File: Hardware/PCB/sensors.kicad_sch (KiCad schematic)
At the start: 26 parts, among them IC3 MPX5500DP, IC4 MPX5500DP, U2 ADS1219IPWR, U6 TPS7A2050PDBVR

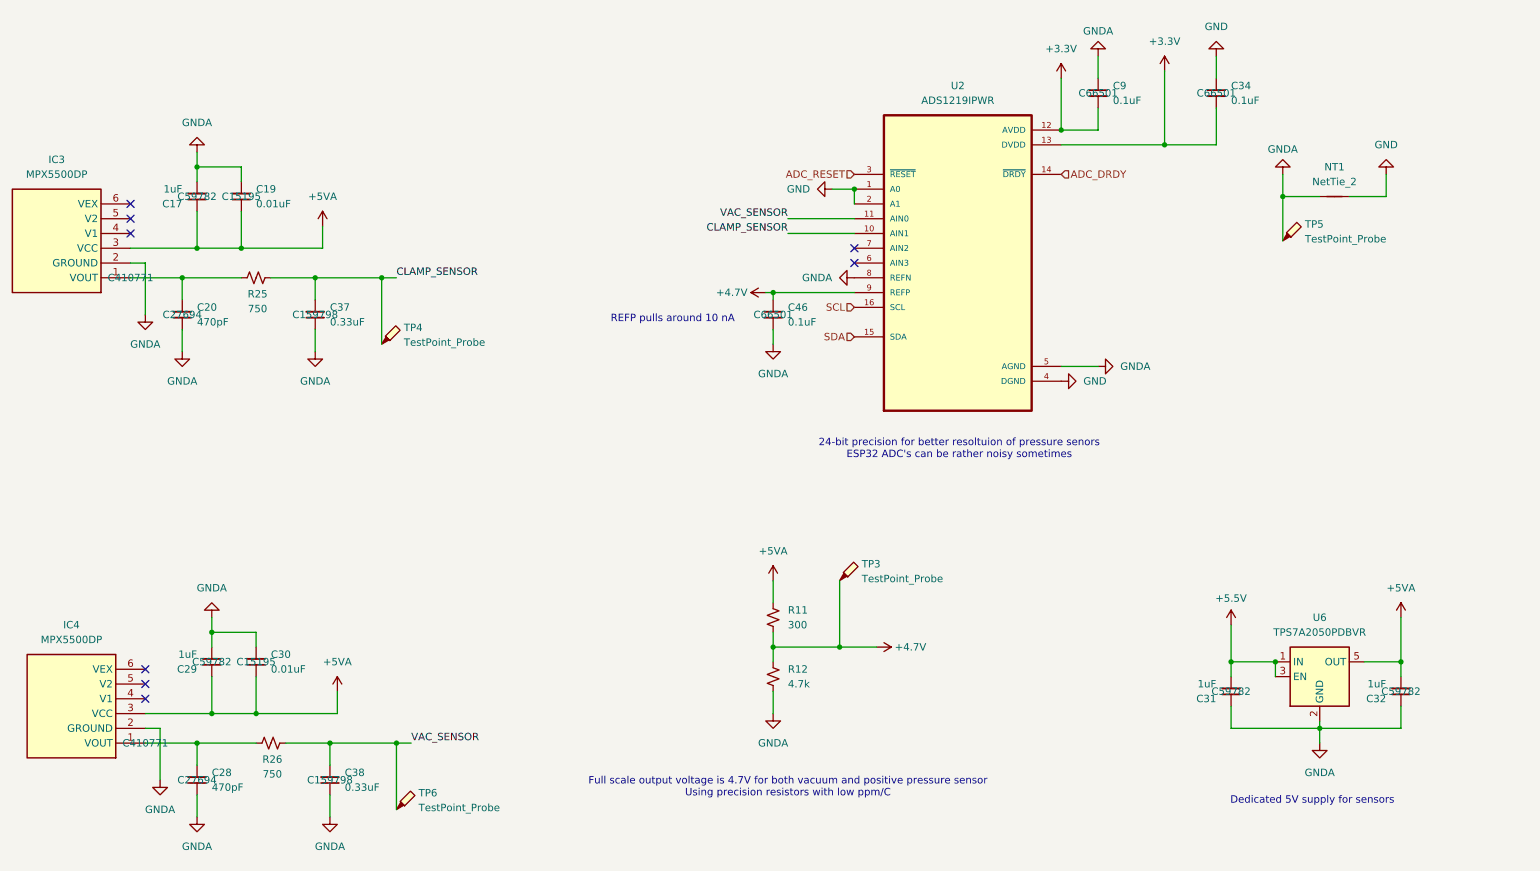
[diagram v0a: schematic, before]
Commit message: done with this, placed order
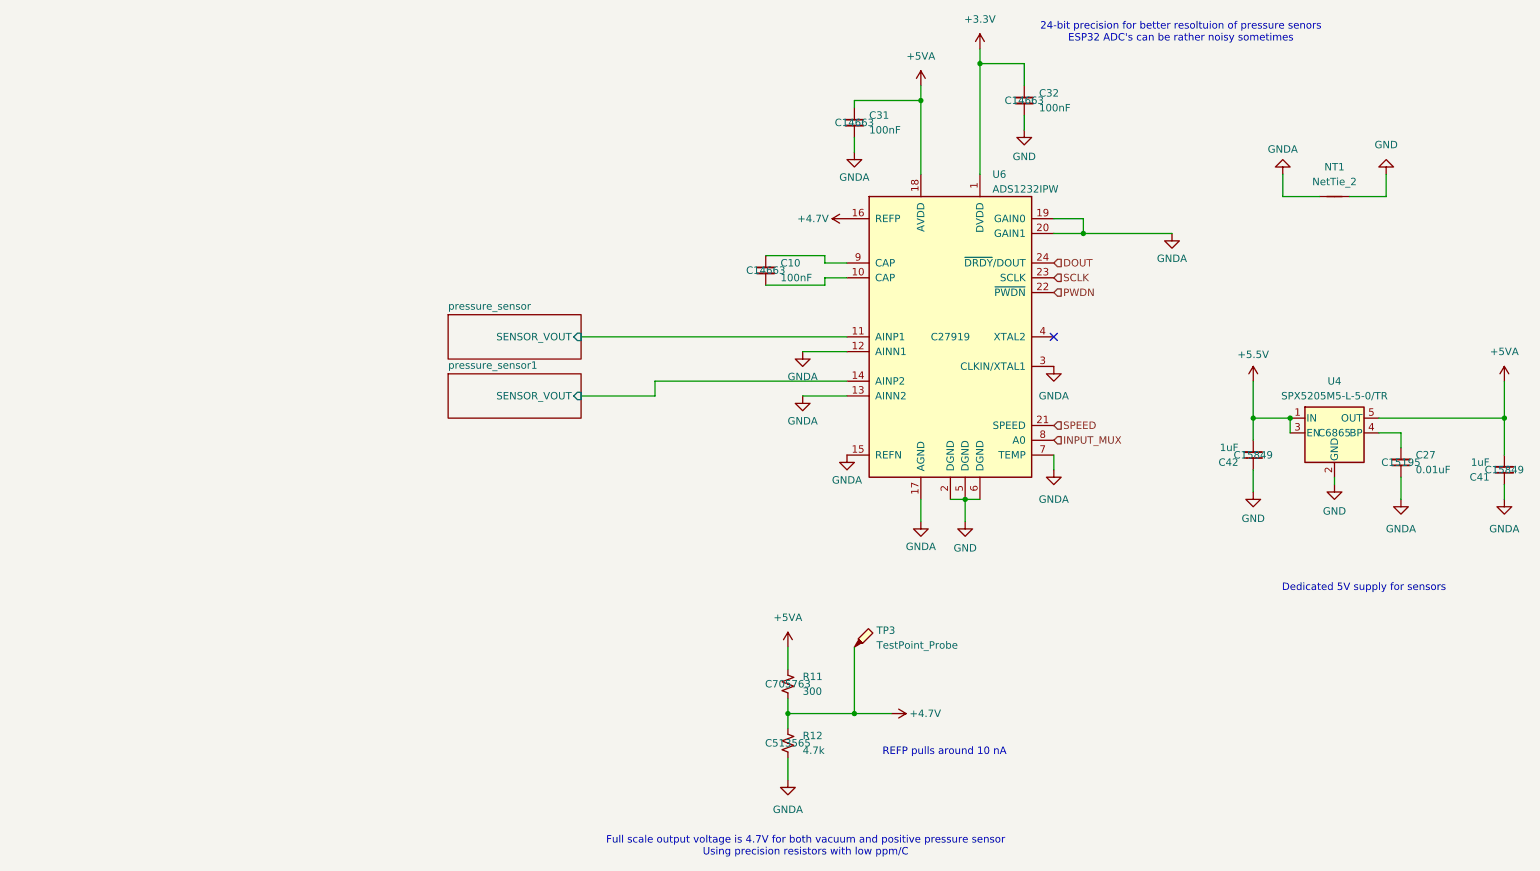
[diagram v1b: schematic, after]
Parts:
- removed C17, C29: 1uF, Capacitor_SMD:C_0603_1608Metric_Pad1.08x0.95mm_HandSolder, symbol Device:C_Small
- removed C19, C30: 0.01uF, Capacitor_SMD:C_0402_1005Metric_Pad0.74x0.62mm_HandSolder, symbol Device:C_Small
- removed C20, C28: 470pF, Capacitor_SMD:C_0603_1608Metric_Pad1.08x0.95mm_HandSolder, symbol Device:C_Small
- removed C34, C46, C9: 0.1uF, Capacitor_SMD:C_0603_1608Metric_Pad1.08x0.95mm_HandSolder, symbol Device:C_Small
- removed C37, C38: 0.33uF, Capacitor_SMD:C_0603_1608Metric_Pad1.08x0.95mm_HandSolder, symbol Device:C_Small
- removed IC3, IC4: MPX5500DP, Vendor_Footprints:MPX5500DP, symbol Vendor_Symbols:MPX5500DP
- removed R25, R26: 750, Resistor_SMD:R_0603_1608Metric_Pad0.98x0.95mm_HandSolder, symbol Device:R_Small_US
- removed TP4, TP5, TP6: TestPoint_Probe, TestPoint:TestPoint_Keystone_5000-5004_Miniature, symbol Connector:TestPoint_Probe
- removed U2: ADS1219IPWR, Vendor_Footprints:SOP65P640X120-16N, symbol Vendor_Symbols:ADS1219IPWR
- removed U6: TPS7A2050PDBVR, Package_TO_SOT_SMD:SOT-23-5, symbol Regulator_Linear:TPS7A0531PDBV
- added C10: 100nF, Capacitor_SMD:C_0603_1608Metric_Pad1.08x0.95mm_HandSolder, symbol Device:C_Small
- added C27: 0.01uF, Capacitor_SMD:C_0402_1005Metric_Pad0.74x0.62mm_HandSolder, symbol Device:C_Small
- added C41, C42: 1uF, Capacitor_SMD:C_0603_1608Metric_Pad1.08x0.95mm_HandSolder, symbol Device:C_Small
- added U4: SPX5205M5-L-5-0/TR, Package_TO_SOT_SMD:SOT-23-5, symbol Regulator_Linear:SPX3819M5-L-5-0
- added U6: ADS1232IPW, Package_SO:TSSOP-24_6.1x7.8mm_P0.65mm, symbol Analog_ADC:ADS1232IPW
- C31, C32: value 1uF -> 100nF; DigiKey Link https://www.digikey.com/en/products/detail/samsung-electro-mechanics/CL10B105KO8NNNC/3886677 -> https://www.digikey.com/en/products/detail/samsung-electro-mechanics/CL10B104KO8NNNC/3886663; LCSC C59782 -> C14663; MPN CL10B105KO8NNNC -> CC0603KRX7R9BB104; Manufacturer Samsung Electro-Mechanics -> YAGEO
- R11: LCSC (none) -> C705763; MPN RG1608P-301-B-T5 -> RT0603BRD07300RL; Manufacturer Susumu -> YAGEO
- R12: LCSC (none) -> C513565; MPN RG1608P-472-B-T5 -> RT0603BRD074K7L; Manufacturer Susumu -> YAGEO
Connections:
- net +3.3V: now also C32.1, U6.1 (DVDD)
- net +4.7V: now also U6.16 (REFP)
- net +5.5V: now also C42.2, U4.1 (IN), U4.3 (EN); no longer C31.2
- net +5VA: now also C31.1, C41.2, U4.5 (OUT), U6.18 (AVDD); no longer C32.2
- net GND: now also C32.2, C42.1, U4.2 (GND), U6.2 (DGND), U6.5 (DGND), U6.6 (DGND)
- net GNDA: now also C31.2, C27.1, C41.1, U6.12 (AINN1), U6.13 (AINN2), U6.15 (REFN), U6.17 (AGND), U6.19 (GAIN0), U6.20 (GAIN1), U6.3 (CLKIN/XTAL1), U6.7 (TEMP); no longer C31.1, C32.1
- new net: C27.2, U4.4 (BP)
- new net: C10.1, U6.9 (CAP)
- new net: C10.2, U6.10 (CAP)
- new net DOUT: U6.24 (~{DRDY}/DOUT)
- new net INPUT_MUX: U6.8 (A0)
- new net PWDN: U6.22 (~{PWDN})
- new net SCLK: U6.23 (SCLK)
- new net SPEED: U6.21 (SPEED)
- new net pressure_sensor/SENSOR_VOUT: U6.11 (AINP1)
- new net pressure_sensor1/SENSOR_VOUT: U6.14 (AINP2)
- no-connect marks 8 -> 1
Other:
- added sheet pressure_sensor (pressure_sensor.kicad_sch)
- added sheet pressure_sensor1 (pressure_sensor.kicad_sch)
- moved on the sheet: R11, R12, TP3
